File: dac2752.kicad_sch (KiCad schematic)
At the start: 30 parts, among them U30 LTC2752B, U301 OPA2197xD, U31 OPA2189D, U32 OPA2388D

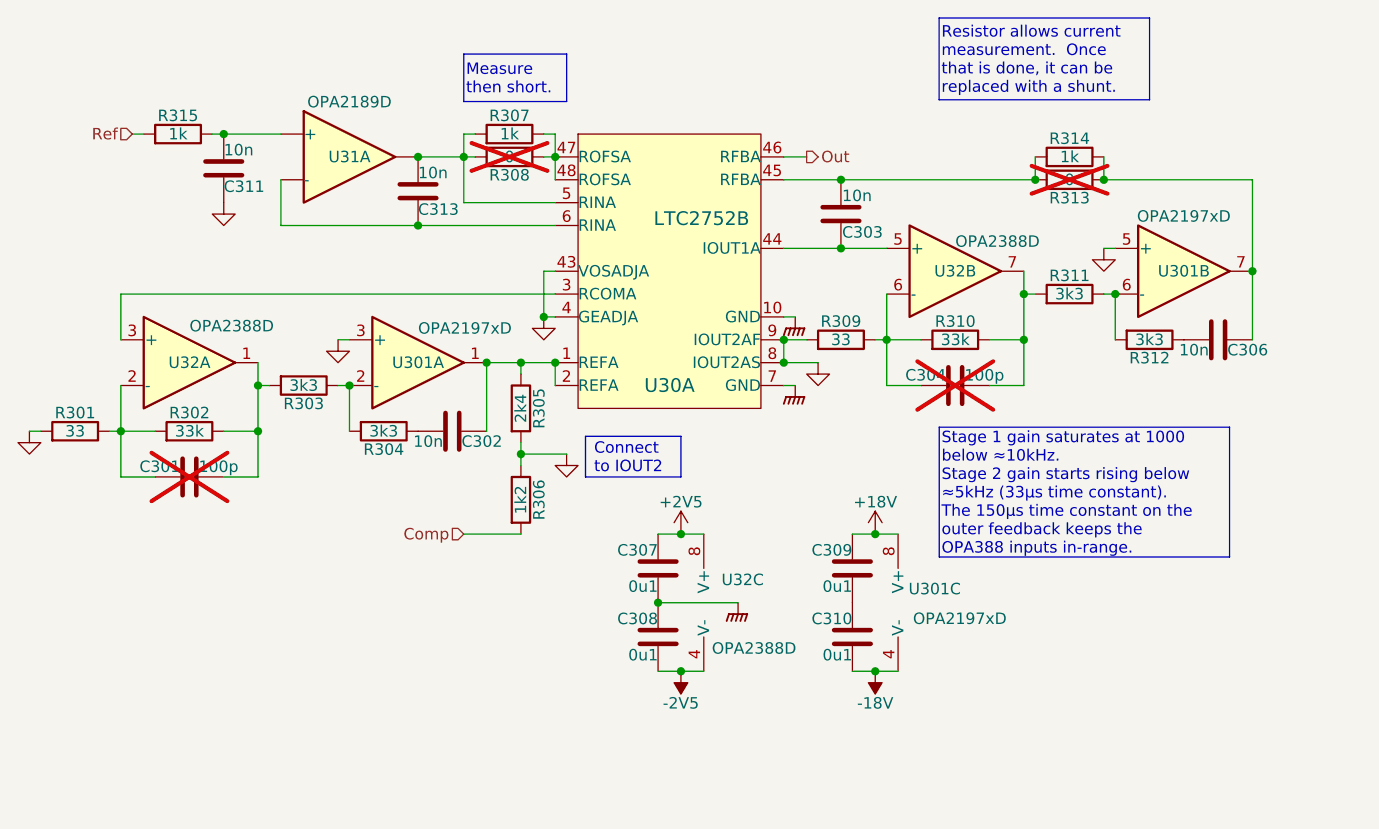
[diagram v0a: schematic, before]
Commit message: ERC passes.
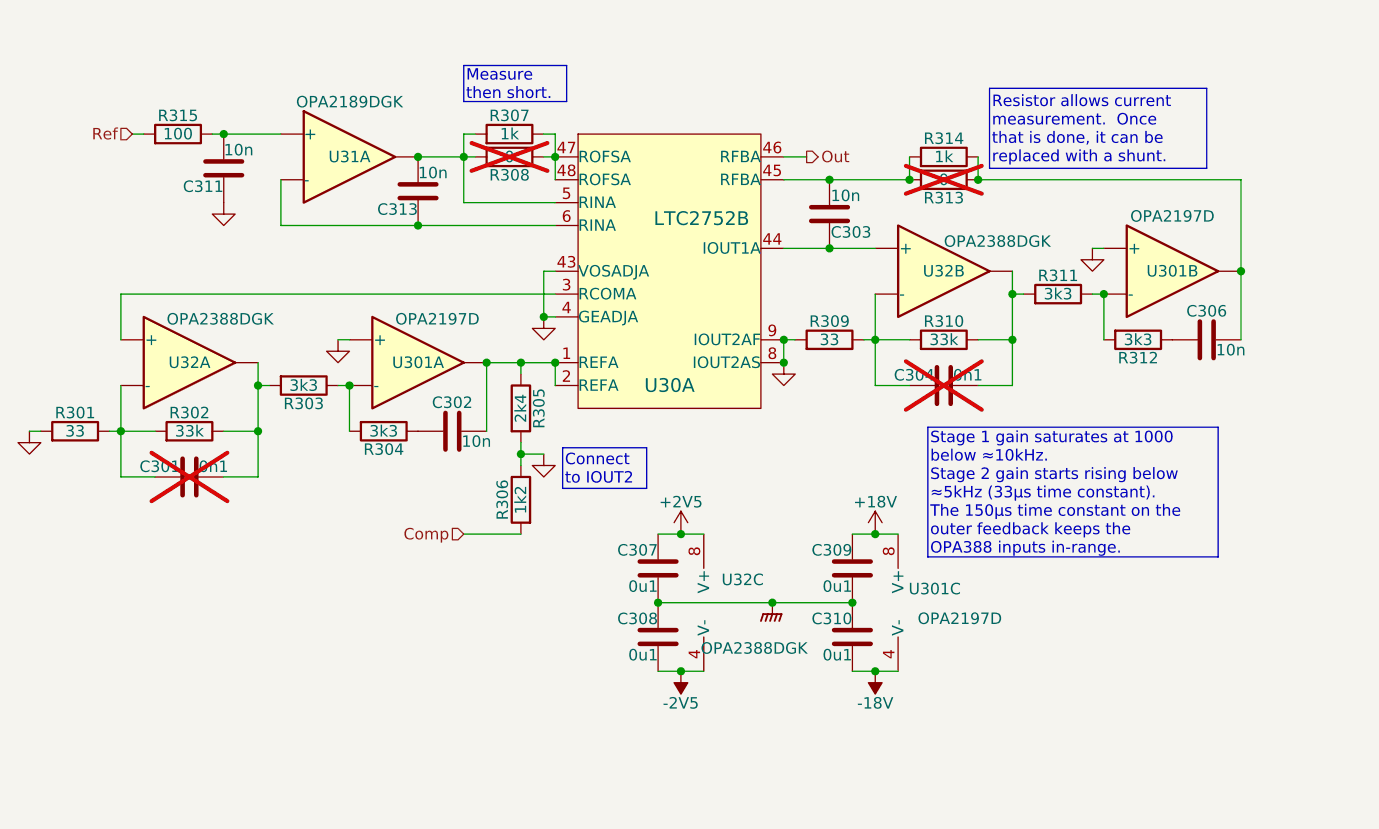
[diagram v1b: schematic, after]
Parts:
- C301, C304: value 100p -> 0n1
- R315: value 1k -> 100; LCSC C11702 -> (none)
- U301: value OPA2197xD -> OPA2197D
- U31: value OPA2189D -> OPA2189DGK; footprint Package_SO:SOIC-8_3.9x4.9mm_P1.27mm -> Package_SO:MSOP-8_3x3mm_P0.65mm; symbol Parts:OPA2189D -> Parts:OPA2189DGK
- U32: value OPA2388D -> OPA2388DGK; footprint Package_SO:SOIC-8_3.9x4.9mm_P1.27mm -> Package_SO:MSOP-8_3x3mm_P0.65mm; symbol Parts:OPA2388D -> Parts:OPA2388DGK; now left out of the parts list
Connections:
- net GNDPWR: now also C309.2, C310.1; no longer U30.10 (GND), U30.7 (GND)
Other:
- moved on the sheet: C303, C304, C306, R309, R310, R311, R312, R313, R314

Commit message: Everything assigned except for wierd shit.
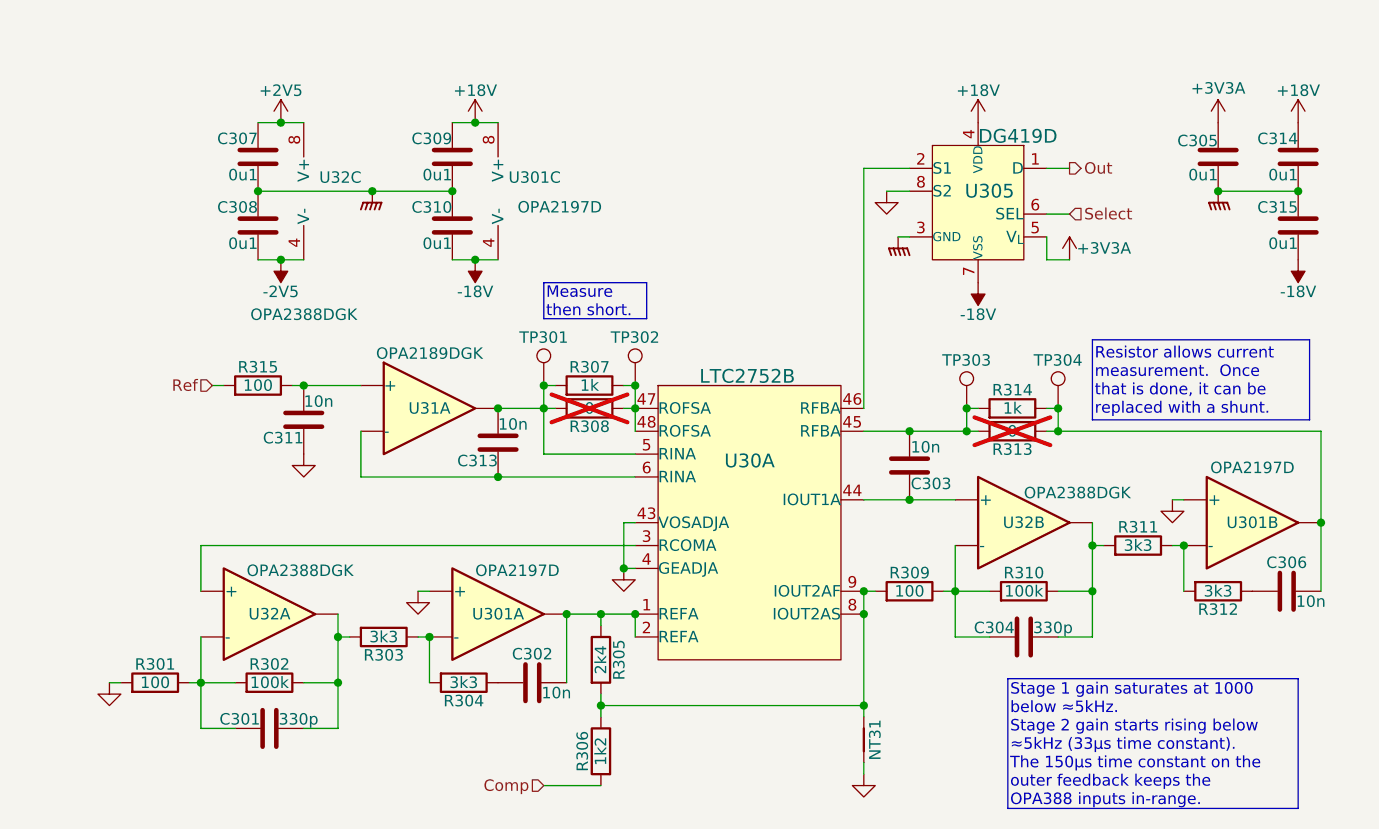
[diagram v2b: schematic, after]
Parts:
- added C305, C314, C315: 0u1, Capacitor_SMD:C_0402_1005Metric, symbol Device:C
- added NT31: NetTie_2, symbol Device:NetTie_2
- added TP301, TP302, TP303, TP304: TestPoint, Parts:TestPoint, symbol Connector:TestPoint
- added U305: DG419D, Package_SO:SOIC-8_3.9x4.9mm_P1.27mm, symbol Parts:DG419
- C301, C304: value 0n1 -> 330p; LCSC (none) -> C1664; now fitted; now in the parts list
- R301, R309: value 33 -> 100
- R302, R310: value 33k -> 100k
- R315: LCSC (none) -> C25076
- U30: LCSC (none) -> C682625
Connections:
- net +18V: now also C314.1, U305.4 (VDD)
- net -18V: now also C315.2, U305.7 (VSS)
- net GND: now also NT31.1, U305.8 (S2); no longer R305.2, R306.1, R309.2, U30.8 (IOUT2AS), U30.9 (IOUT2AF)
- net GNDPWR: now also C305.2, C314.2, C315.1, U305.3 (GND)
- net Out: now also U305.1 (D); no longer U30.46 (RFBA)
- net at C306.1, R313.1, R314.1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: now also TP304.1
- net at C303.1, R313.2, R314.2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: now also TP303.1
- net at R307.1, R308.1, U30.47 (ROFSA)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: now also TP302.1
- net at C313.1, R307.2, R308.2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: now also TP301.1
- new net: U30.46 (RFBA), U305.2 (S1)
- new net: NT31.2, R305.2, R306.1, R309.2, U30.8 (IOUT2AS), U30.9 (IOUT2AF)
- new net +3V3A: C305.1, U305.5 (V_{L})
- new net Select: U305.6 (SEL)
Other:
- moved on the sheet: C302, C303, C306, C307, C308, C309, C310, C311, C313, R301, R302, R303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
